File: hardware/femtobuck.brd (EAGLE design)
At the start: 10.1 x 31.1 mm, 11 parts

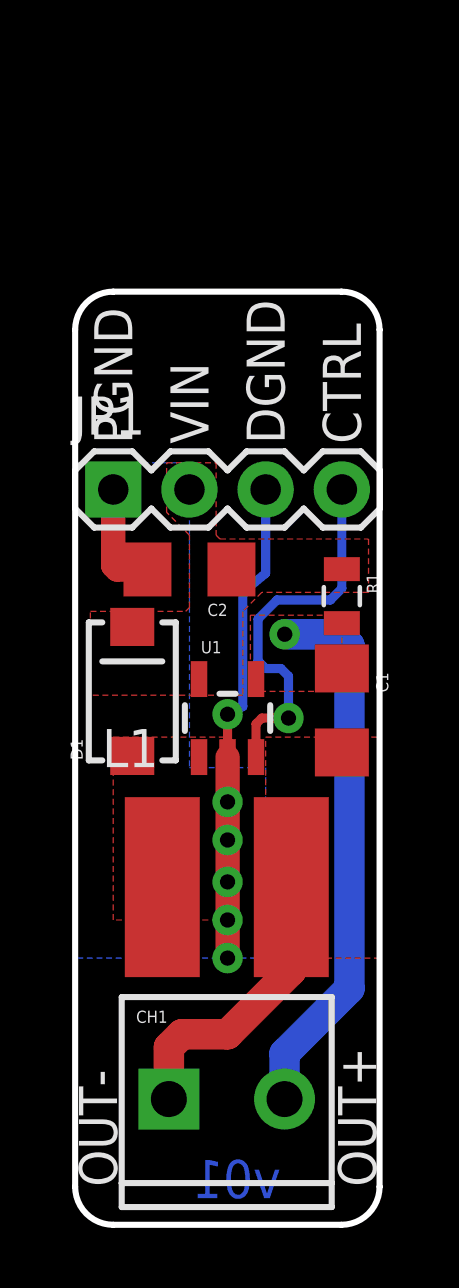
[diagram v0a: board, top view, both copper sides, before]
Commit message: Incorporate changes from review
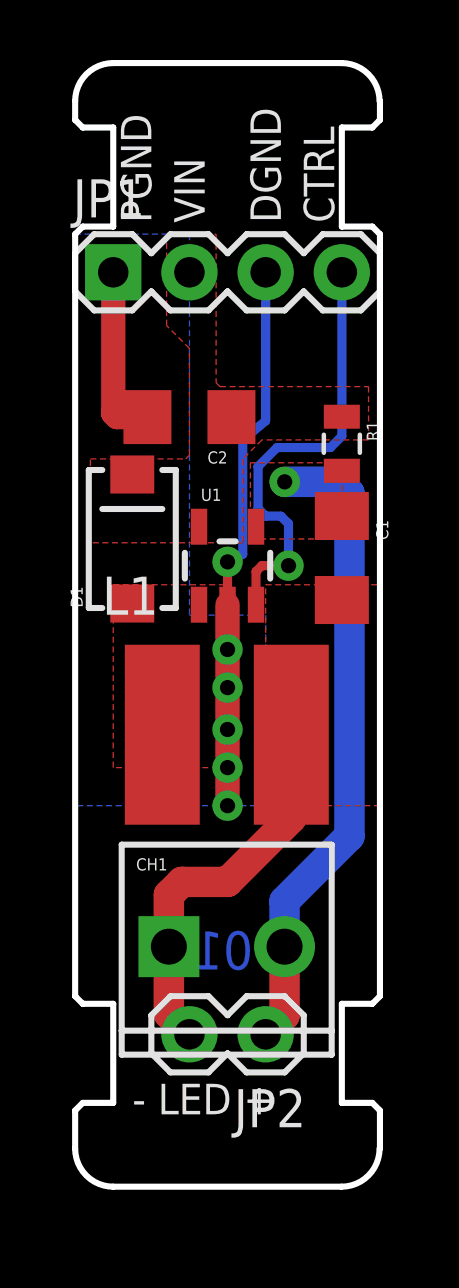
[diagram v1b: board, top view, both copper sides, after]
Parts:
- added JP2: M02PTH, SparkFun-Connectors:1X02
- moved FRAME1 10.2 mm to (11.4, -20.3)
- moved JP1 7.24 mm to (1.27, 31.8)
- moved LOGO2 7.17 mm to (9.78, 24.4)
- moved C1 5.08 mm to (8.89, 22.2)
- moved L1 5.08 mm to (5.08, 16.5)
- moved LOGO1 5.08 mm to (2.03, 26.3)
- moved R1 5.08 mm to (8.89, 26.0)
- moved U1 5.08 mm to (5.08, 22.0)
- moved CH1 5.08 mm to (3.30, 9.27)
- moved C2 5.08 mm to (3.81, 26.9)
- moved D1 5.08 mm to (1.91, 22.9)
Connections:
- net OUT+: now also JP2.1
- net OUT-: now also JP2.2
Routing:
- net GND: track 19.9 -> 24.2 mm
- net OUT-: track 9.65 -> 12.9 mm
- net OUT+: track 18.3 -> 21.5 mm
- net CTRL_CH1: track 12.8 -> 15.0 mm
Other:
- board size 10.1 x 31.1 mm -> 10.2 x 37.5 mm
- board text added: "+ LED -"
- board text added: "- LED +"
- board text added: "M. Hord"
- board text removed: "M. Hord/E. Zonca"
- board text removed: "OUT+"
- board text removed: "OUT-"
